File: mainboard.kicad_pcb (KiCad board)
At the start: 2 copper layers, 90 x 120 mm, 29 parts, among them J1 terminal_led-strip, J2 header_rotary-encoder, J4 header_pi, J5 power_input, J6 AudioJack2, Q1 IRF9540N, SW1 power_switch, U1 OPA2277, U2 MSGEQ7, U4 logic-level-converter, U5 logic-level-converter

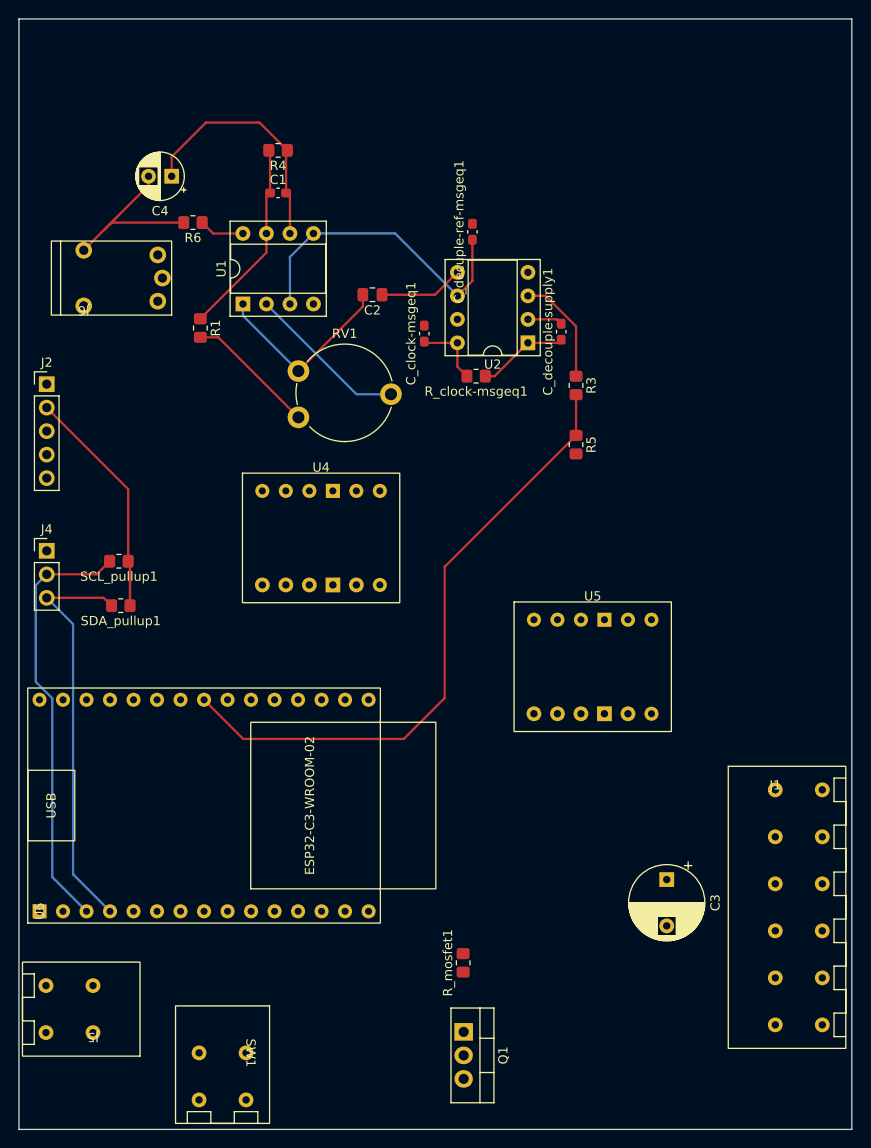
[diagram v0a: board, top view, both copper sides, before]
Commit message: route tracks and add mounting holes
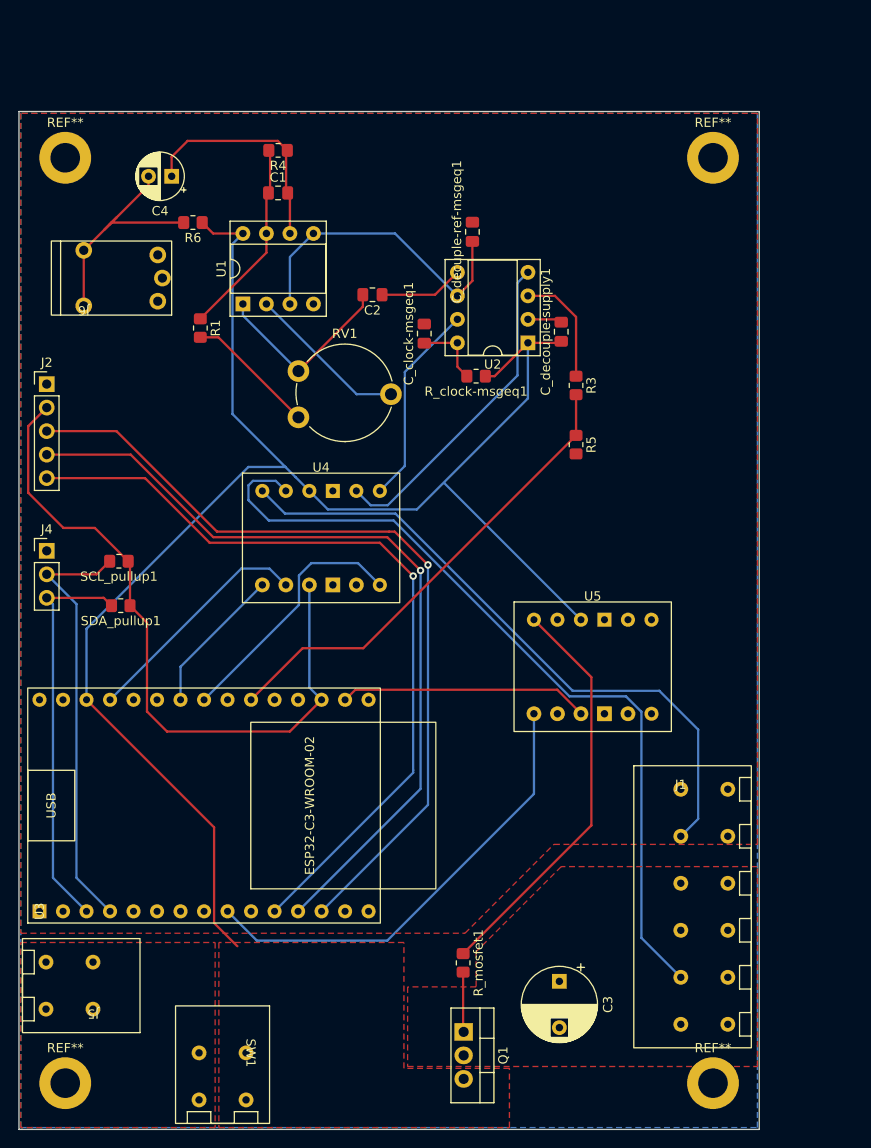
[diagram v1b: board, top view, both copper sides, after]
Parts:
- removed U6: ~, my_lib:esp32_c3_dev-kit-c_02
- added REF**: MountingHole_3.2mm_M3_DIN965_Pad, MountingHole:MountingHole_3.2mm_M3_DIN965_Pad, F.Cu at (125.0, 65.0)
- added REF**: MountingHole_3.2mm_M3_DIN965_Pad, MountingHole:MountingHole_3.2mm_M3_DIN965_Pad, F.Cu at (55.0, 165.0)
- added REF**: MountingHole_3.2mm_M3_DIN965_Pad, MountingHole:MountingHole_3.2mm_M3_DIN965_Pad, F.Cu at (125.0, 165.0)
- added REF**: MountingHole_3.2mm_M3_DIN965_Pad, MountingHole:MountingHole_3.2mm_M3_DIN965_Pad, F.Cu at (55.0, 65.0)
- added U3: ~, my_lib:esp32_c3_dev-kit-c_02, F.Cu at (52.2, 146.4)
- C1, C_clock-msgeq1, C_decouple-supply1, C_decuple-ref-msgeq1: footprint Capacitor_SMD:C_0603_1608Metric_Pad1.08x0.95mm_HandSolder -> Capacitor_SMD:C_0805_2012Metric_Pad1.18x1.45mm_HandSolder
- moved C3 16.0 mm to (108.4, 154.0)
- moved J1 10.2 mm to (121.5, 133.2)
- moved J5 2.54 mm to (58.0, 157.0)
- turned R_mosfet1 to -90 degrees
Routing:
- net 5V: track 15.0 -> 172.8 mm
- net rotary_sw: track 0.00 -> 89.4 mm, vias 0 -> 1
- net Net-(J1-Pin_5): track 0.00 -> 88.7 mm
- net rotary_dt: track 0.00 -> 87.9 mm, vias 0 -> 1
- net rotary_clk: track 0.00 -> 86.4 mm, vias 0 -> 1
- net 3V3: track 25.1 -> 102.1 mm
- net Net-(J1-Pin_2): track 0.00 -> 70.1 mm
- net Net-(U3-GPIO10): track 0.00 -> 49.7 mm
- net power_fet: track 0.00 -> 44.4 mm
- net msgeq7-strobe: track 0.00 -> 35.5 mm
- net esp_msgeq7-reset: track 0.00 -> 28.0 mm
- net esp_led-strip_back: track 0.00 -> 25.6 mm
- net msgeq7-reset: track 0.00 -> 22.0 mm
- net Net-(U3-GPIO4/ADC1_CH4): track 68.3 -> 51.4 mm
- net esp_led-strip_front: track 0.00 -> 16.1 mm
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- added copper zone on F.Cu, net +5V
- added copper zone on F.Cu, net 5V
- added copper zone on F.Cu, net 5V_led
- added copper zone on B.Cu, net GND
- added copper zone on F.Cu, net GND
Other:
- board size 90 x 120 mm -> 80 x 110 mm
